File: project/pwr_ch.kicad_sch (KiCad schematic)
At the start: 16 parts, among them J201 XT-IN, J202 METER, J203 XT-OUT, Q201 AON6144, U201 UCC27517DBVR

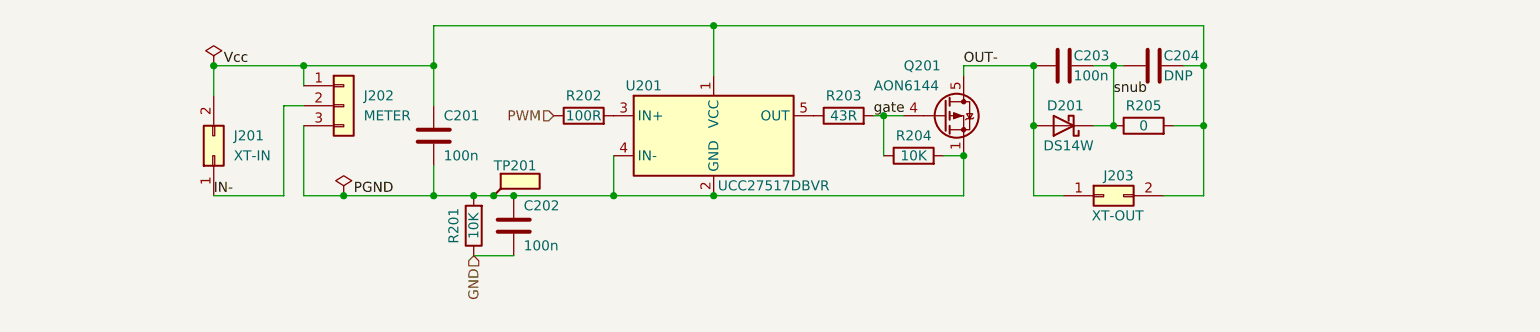
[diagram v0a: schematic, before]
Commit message: fixing a lot of stuff in power board
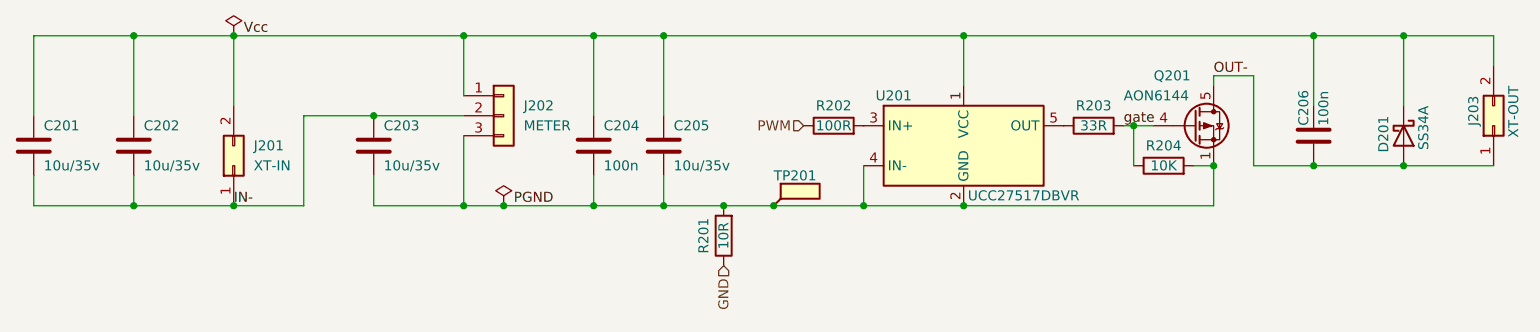
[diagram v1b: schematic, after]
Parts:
- removed C204: DNP, Capacitor_SMD:C_0805_2012Metric_Pad1.18x1.45mm_HandSolder, symbol Device:C
- removed R205: 0, Resistor_SMD:R_0805_2012Metric_Pad1.20x1.40mm_HandSolder, symbol Device:R
- added C201, C203, C205: 10u/35v, Capacitor_SMD:C_1206_3216Metric_Pad1.33x1.80mm_HandSolder, symbol Device:C
- C202: value 100n -> 10u/35v; footprint Capacitor_SMD:C_0805_2012Metric_Pad1.18x1.45mm_HandSolder -> Capacitor_SMD:C_1206_3216Metric_Pad1.33x1.80mm_HandSolder; lcsc# C476766 -> C92797
- D201: value DS14W -> SS34A; footprint Diode_SMD:D_SOD-123F -> Diode_SMD:D_SMA; lcsc# C1884542 -> C2886580
- R201: value 10K -> 10R
- R203: value 43R -> 33R
- renumbered C201 to C204, C203 to C206
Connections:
- net snub is gone; now on net Vcc: C206.1, D201.1 (K)
- net GND: no longer C202.2
- net IN-: now also C202.2, C201.2, C203.1
- net PGND: now also C203.2, C205.2; no longer C202.1
- net Vcc: now also C202.1, C201.1, C205.1
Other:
- moved on the sheet: C204, C206, J201, J202, J203, Q201, R201, R202, R203, R204, TP201, U201
